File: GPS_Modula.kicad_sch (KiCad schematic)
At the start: 16 parts, among them U11 AMS1117-3.3, U2 NEO-M8M, U5 AT24CS01-XHM

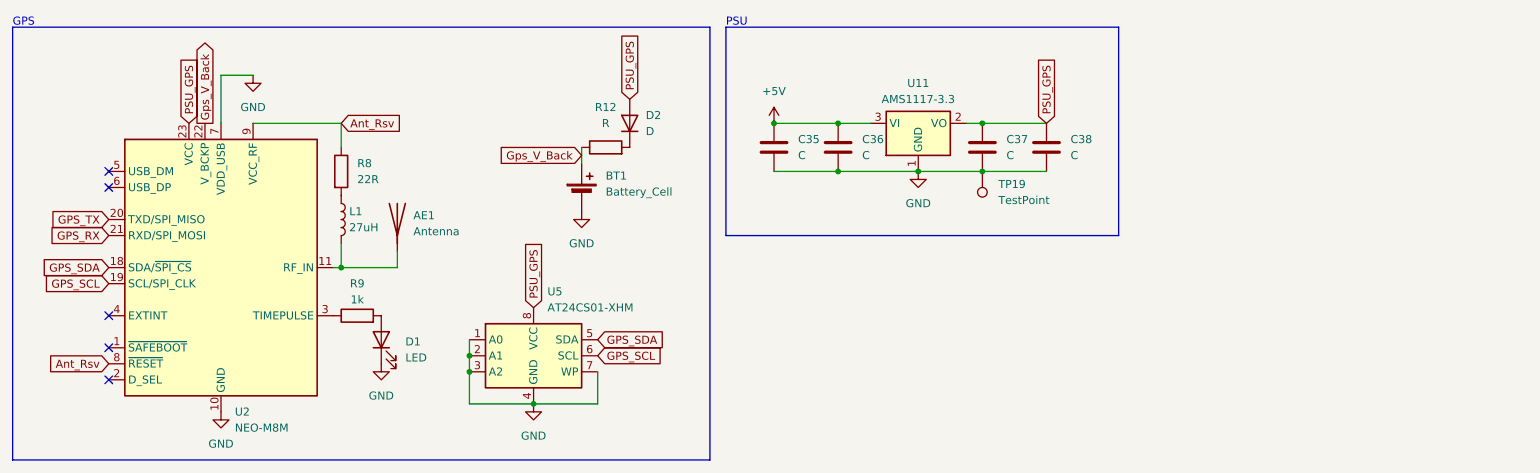
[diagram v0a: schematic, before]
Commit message: done most of the schematics
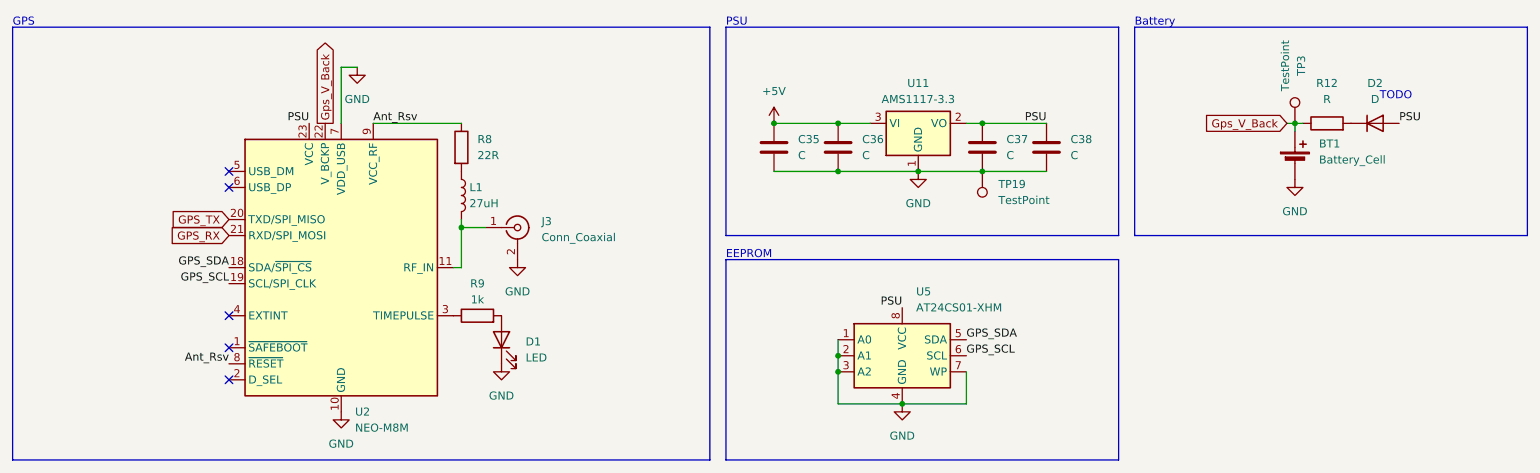
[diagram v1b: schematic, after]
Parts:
- removed AE1: Antenna, symbol Device:Antenna
- added J3: Conn_Coaxial, symbol Connector:Conn_Coaxial
- added TP3: TestPoint, symbol Connector:TestPoint
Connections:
- net GND: now also J3.2 (Ext)
- net Gps_V_Back: now also TP3.1
- net at L1.2, U2.11 (RF_IN): now also J3.1 (In)
- net PSU_GPS renamed PSU
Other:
- note added: "Battery"
- note added: "EEPROM"
- note added: "TODO"
- moved on the sheet: BT1, D1, D2, L1, R12, R8, R9, U2, U5
